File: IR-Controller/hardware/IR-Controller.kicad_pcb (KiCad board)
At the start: 2 copper layers, 40.1 x 80.1 mm, 12 parts, among them J1 Conn_1x06_Generic, Q1 MMBT3904LT1G, SW1 MCSLPT4644B1TR, SW2 MCSLPT4644B1TR, U1 PIC18LF2550-ISO

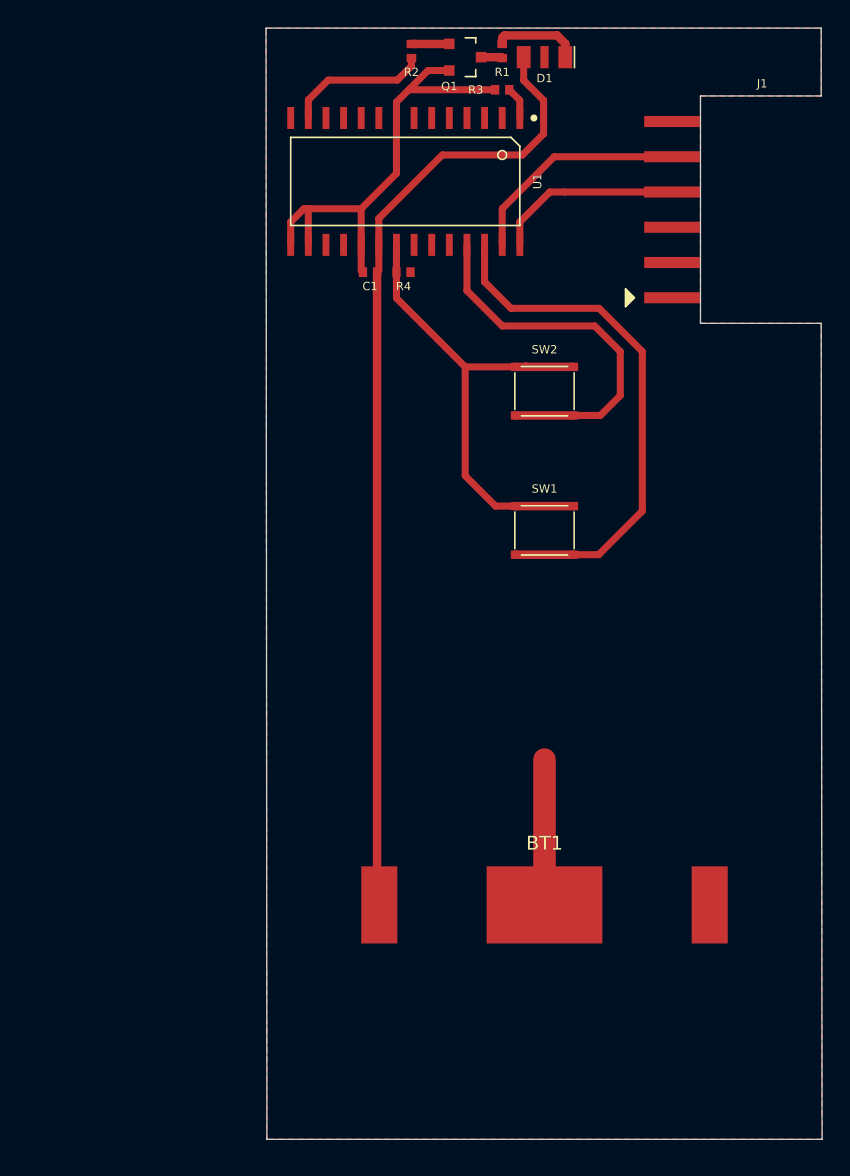
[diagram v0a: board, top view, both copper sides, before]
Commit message: Update exports
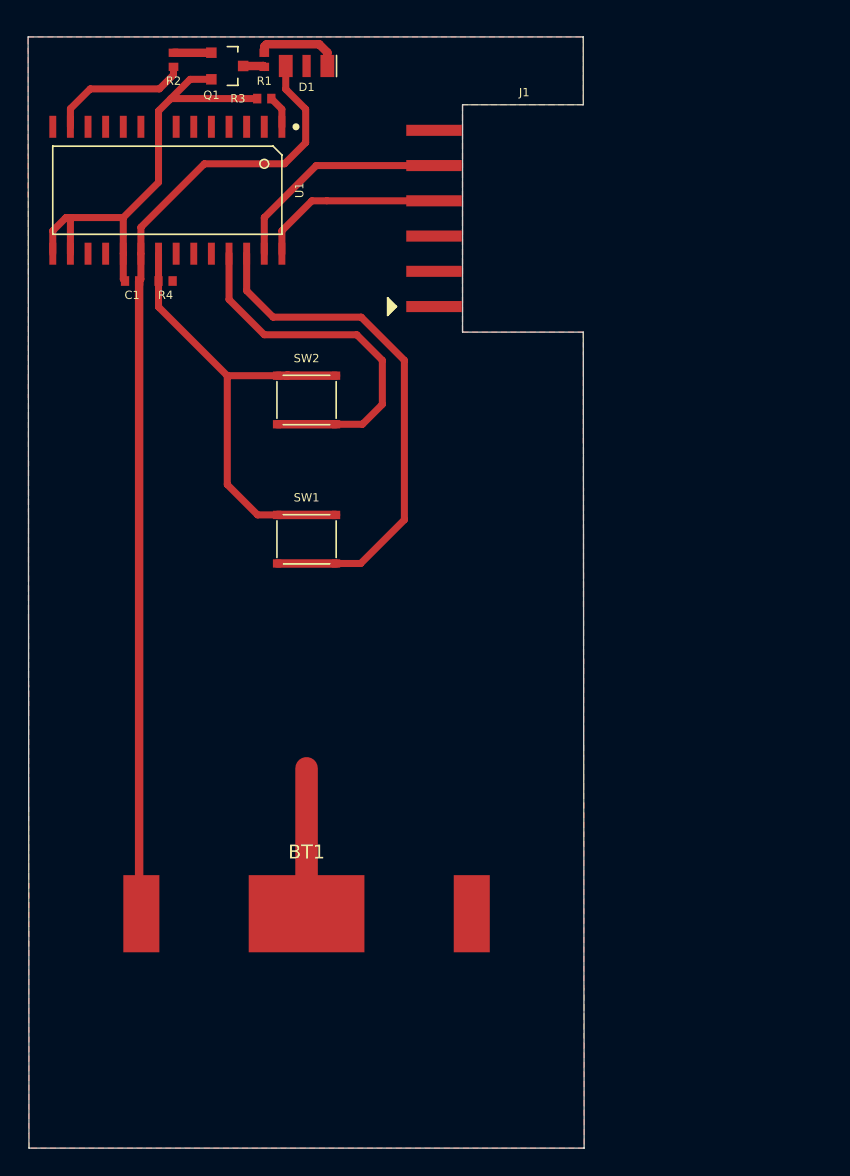
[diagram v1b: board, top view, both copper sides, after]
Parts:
- moved BT1 17.2 mm to (150.4, 119.7)
- moved C1 17.2 mm to (137.8, 74.1)
- moved D1 17.2 mm to (150.4, 58.6)
- moved Q1 17.2 mm to (144.7, 58.6)
- moved R1 17.2 mm to (147.3, 58.2)
- moved R3 17.2 mm to (147.3, 61.0)
- moved R4 17.2 mm to (140.2, 74.1)
- moved SW1 17.2 mm to (150.4, 92.7)
- moved SW2 17.2 mm to (150.4, 82.7)
- moved J1 17.2 mm to (166.1, 69.6)
- moved R2 17.2 mm to (140.8, 58.2)
- moved U1 17.2 mm to (140.3, 67.6)
